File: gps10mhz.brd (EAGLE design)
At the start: 100 x 80 mm, 28 parts, among them IC2 7803.3, IC3 CD74HC132E, U1 BB3553AM

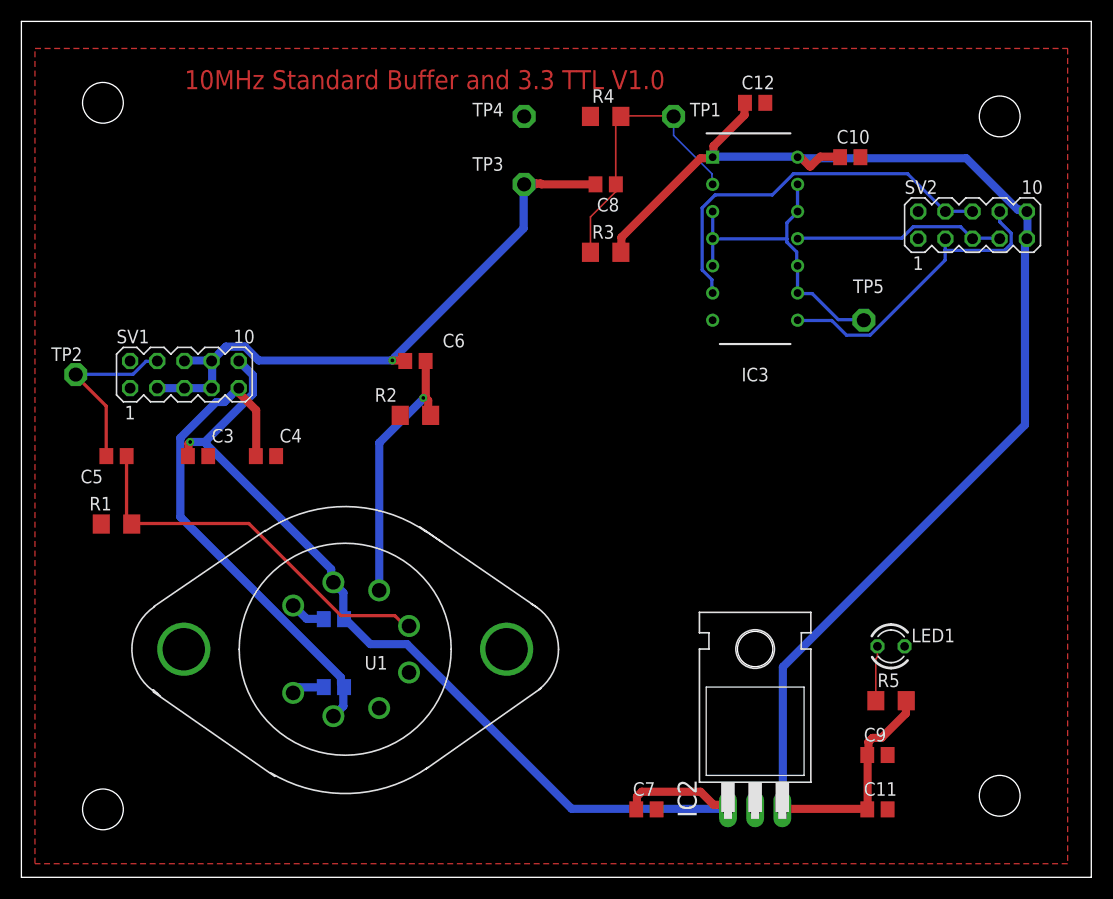
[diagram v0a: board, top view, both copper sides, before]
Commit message: up
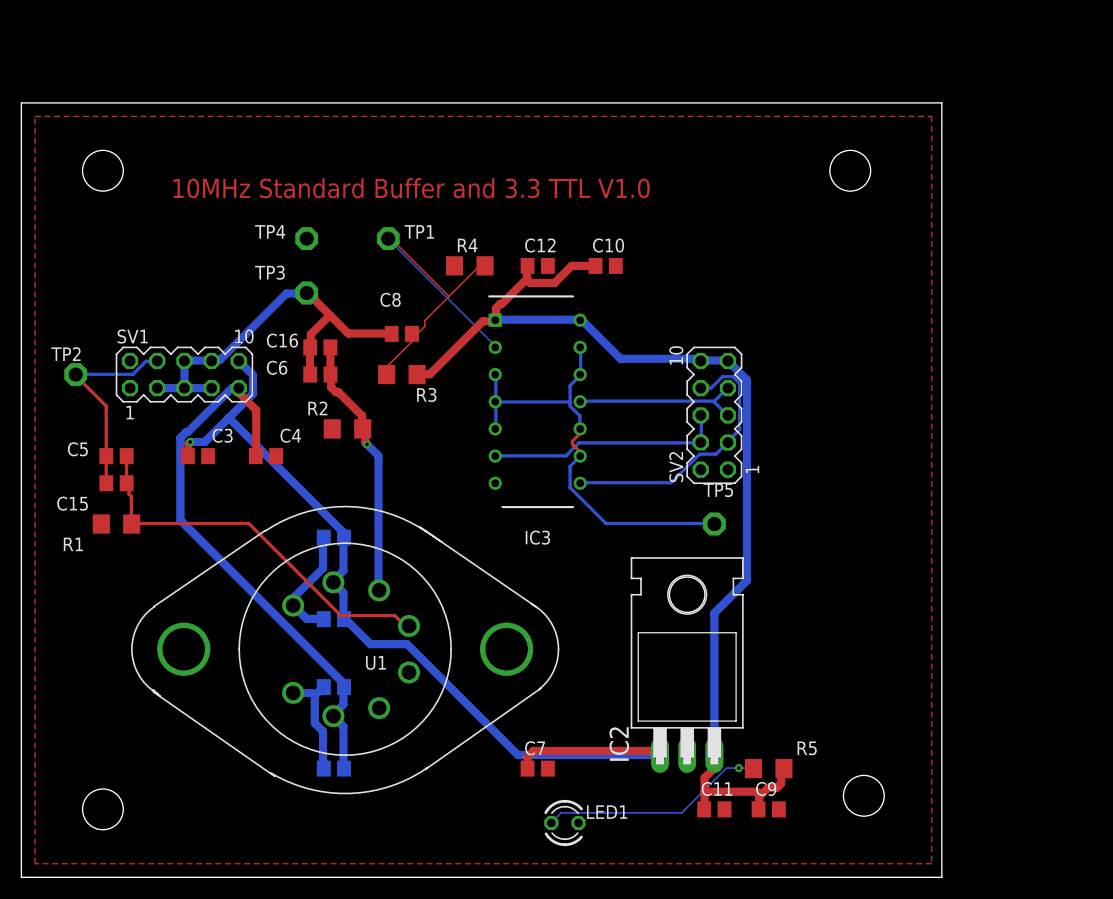
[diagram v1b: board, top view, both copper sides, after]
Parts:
- added C13, C14, C15, C16: 0.01uf, rcl:C0805
- moved LED1 34.7 mm to (50.8, 5.08)
- moved SV2 30.0 mm to (64.8, 43.2), turned to 90 degrees
- moved TP1 29.0 mm to (34.3, 59.7)
- moved C12 25.4 mm to (48.3, 57.1)
- moved IC3 25.4 mm to (48.3, 44.5)
- moved C10 25.0 mm to (54.6, 57.1)
- moved C8 23.6 mm to (35.6, 50.8)
- moved TP5 23.6 mm to (64.8, 33.0)
- moved TP4 23.3 mm to (26.7, 59.7)
- moved TP3 22.7 mm to (26.7, 54.6)
- moved R3 22.2 mm to (35.6, 47.0)
- moved R4 18.9 mm to (41.9, 57.1)
- moved C11 15.2 mm to (64.8, 6.35)
- moved R5 13.1 mm to (69.8, 10.2)
- moved C9 11.4 mm to (69.8, 6.35)
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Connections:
- net +15V: now also C14.1
- net -15V: now also C13.1
- net 0V: now also C13.2, C14.2
- net 10MHZ_IN: now also C15.2
- net 10MHZ_OUT: now also C16.1
- net IN: now also C15.1
- net OUT: now also C16.2
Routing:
- net +3V3: track 141.1 -> 101.4 mm
- net 10MHZ_OUT: track 57.8 -> 37.6 mm, vias 1 -> 0
- net N$1: track 5.14 -> 21.1 mm, vias 0 -> 1
- net 0V: track 6.46 -> 21.3 mm
- net N$2: track 36.4 -> 22.3 mm
- net TTL: track 30.3 -> 42.1 mm
- net SINE_IN: track 26.8 -> 36.8 mm
- net -15V: track 47.2 -> 52.5 mm
- net N$4: track 19.9 -> 16.2 mm
- net N$3: track 29.2 -> 25.7 mm
- net +15V: track 88.5 -> 85.5 mm
- net 10MHZ_IN: track 17.0 -> 19.5 mm
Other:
- board size 100 x 80 mm -> 86 x 72.4 mm
